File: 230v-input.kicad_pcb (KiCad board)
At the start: 2 copper layers, 61.5 x 19.8 mm, 7 parts, among them J1 PWR_IN, U1 MOC3063M, U2 LTV-814

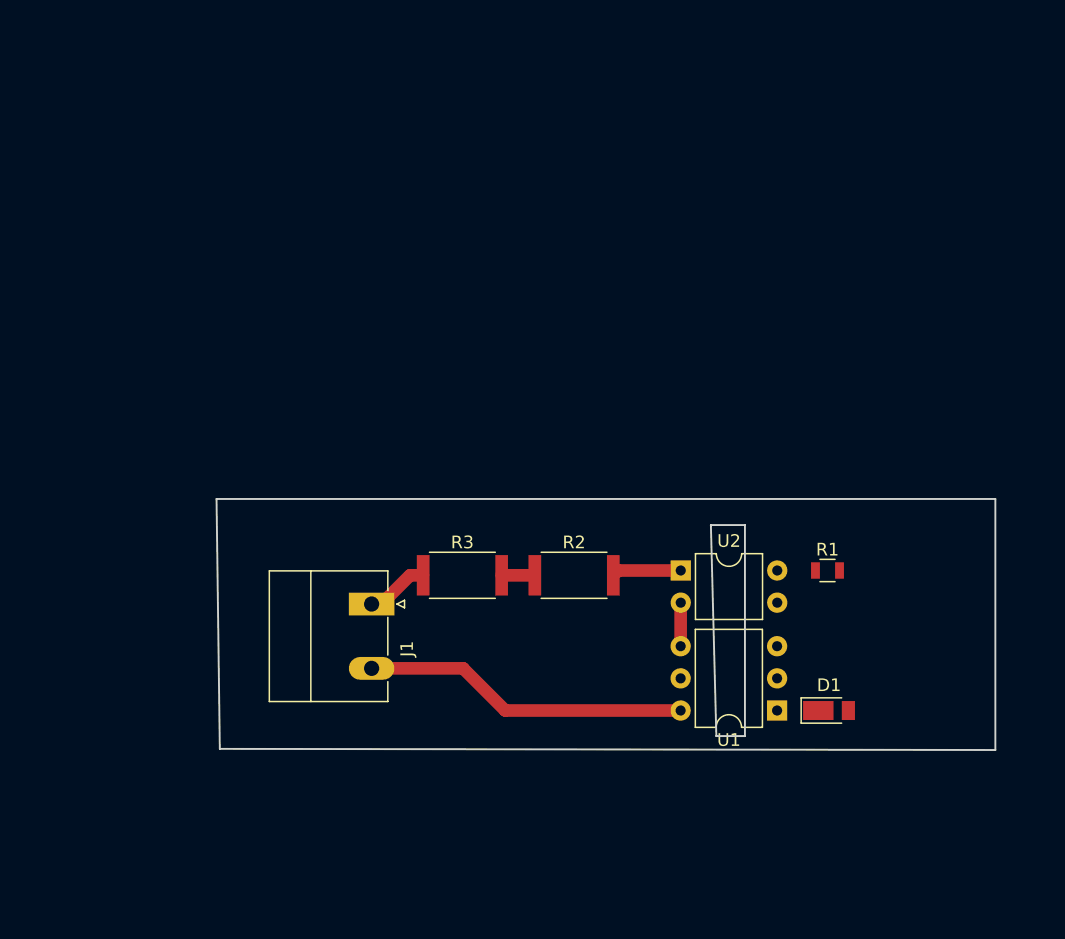
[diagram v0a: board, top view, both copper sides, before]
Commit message: Finish first rev
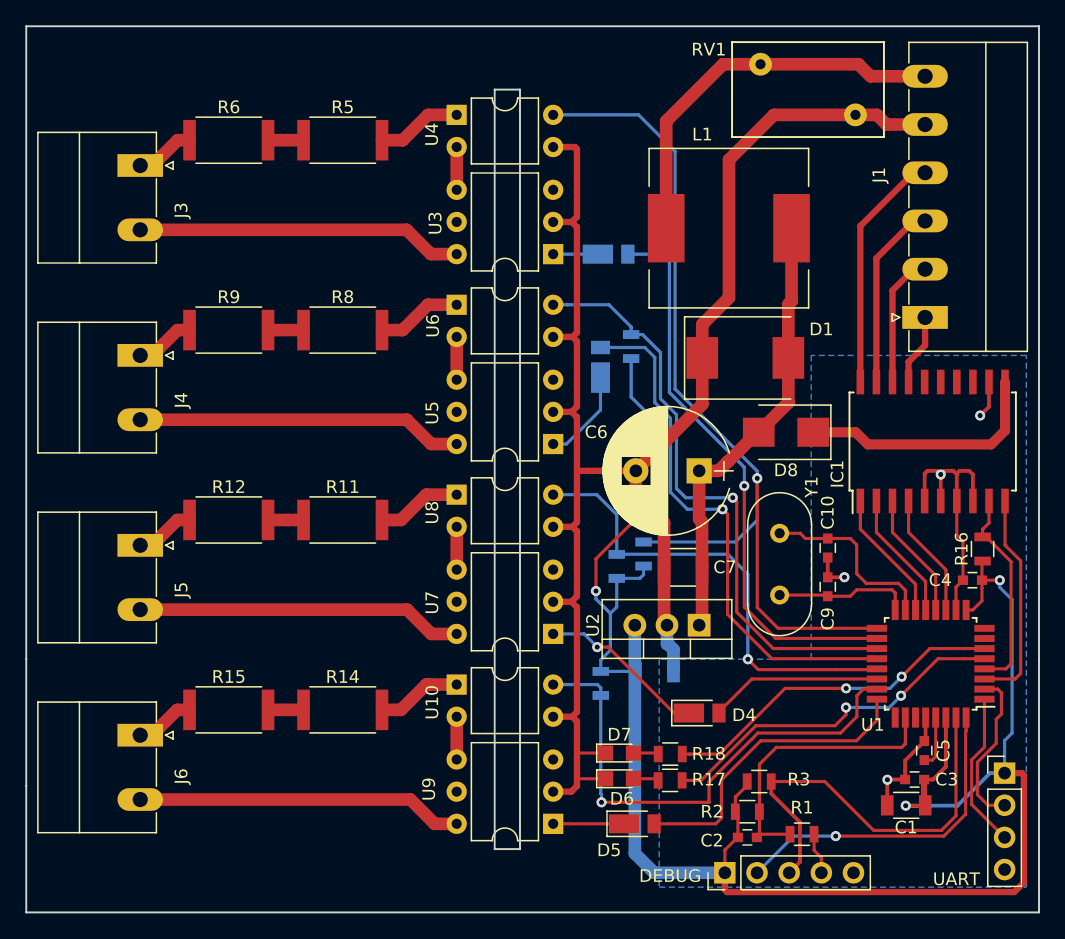
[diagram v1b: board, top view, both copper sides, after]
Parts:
- added C1: 10µF/10V, Capacitors_SMD:C_1206, F.Cu at (89.5, 81.5)
- added C10: 22pF, Capacitors_SMD:C_0603, F.Cu at (83.3, 61.2)
- added C2: 100pF, Capacitors_SMD:C_0603, F.Cu at (77.0, 84.1)
- added C3: 100nF, Capacitors_SMD:C_0603, F.Cu at (90.2, 79.5)
- added C4: 100nF, Capacitors_SMD:C_0603, F.Cu at (94.7, 63.8)
- added C5: 100nF, Capacitors_SMD:C_0603, F.Cu at (90.9, 77.2)
- added C6: 220µF/50V, Capacitors_THT:CP_Radial_D10.0mm_P5.00mm, F.Cu at (73.2, 55.1)
- added C7: 10µF/50V, Capacitors_SMD:C_1210, F.Cu at (71.9, 62.7)
- added C8: 10µF/10V, Capacitors_SMD:C_1206, B.Cu at (69.6, 71.0)
- added C9: 22pF, Capacitors_SMD:C_0603, F.Cu at (83.3, 64.3)
- added D2: AL5809-15, Diodes_SMD:D_PowerDI-123, B.Cu at (66.0, 38.0)
- added D3: AL5809-15, Diodes_SMD:D_PowerDI-123, B.Cu at (65.4, 46.9)
- added D4: AL5809-15, Diodes_SMD:D_PowerDI-123, F.Cu at (73.2, 74.2)
- added D5: AL5809-15, Diodes_SMD:D_PowerDI-123, F.Cu at (68.1, 83.0)
- added D6: LED_RD, LEDs:LED_0805, F.Cu at (66.9, 79.4)
- added D7: LED_GN, LEDs:LED_0805, F.Cu at (66.9, 77.4)
- added D8: STPS3L60U, Diodes_SMD:D_SMB, F.Cu at (80.0, 52.1)
- added IC1: UDN2987, Housings_SOIC:SOIC-20W_7.5x12.8mm_Pitch1.27mm, F.Cu at (91.6, 52.8)
- added J2: DEBUG, Pin_Headers:Pin_Header_Straight_1x05_Pitch2.54mm, F.Cu at (75.2, 86.9)
- added J3: PWR_IN, Connectors_Phoenix:PhoenixContact_MC-G_02x5.08mm_Angled, F.Cu at (29.0, 31.0)
- added J4: PWR_IN, Connectors_Phoenix:PhoenixContact_MC-G_02x5.08mm_Angled, F.Cu at (29.0, 46.0)
- added J5: PWR_IN, Connectors_Phoenix:PhoenixContact_MC-G_02x5.08mm_Angled, F.Cu at (29.0, 61.0)
- added J6: PWR_IN, Connectors_Phoenix:PhoenixContact_MC-G_02x5.08mm_Angled, F.Cu at (29.0, 76.0)
- added J7: UART, Pin_Headers:Pin_Header_Straight_1x04_Pitch2.54mm, F.Cu at (97.3, 79.0)
- added L1: DE1207-82, Inductors_SMD:L_12x12mm_h8mm, F.Cu at (75.5, 36.0)
- added R10: 4k7, Resistors_SMD:R_0805, B.Cu at (66.6, 62.7)
- added R11: 12k/1W, Resistors_SMD:R_2512, F.Cu at (45.0, 59.0)
- added R12: 12k/1W, Resistors_SMD:R_2512, F.Cu at (36.0, 59.0)
- added R13: 4k7, Resistors_SMD:R_0805, B.Cu at (65.4, 71.9)
- added R14: 12k/1W, Resistors_SMD:R_2512, F.Cu at (45.0, 74.0)
- added R15: 12k/1W, Resistors_SMD:R_2512, F.Cu at (36.0, 74.0)
- added R16: 10k, Resistors_SMD:R_0805, F.Cu at (95.5, 61.3)
- added R17: 470, Resistors_SMD:R_0805, F.Cu at (70.9, 79.6)
- added R18: 470, Resistors_SMD:R_0805, F.Cu at (70.9, 77.5)
- added R4: 4k7, Resistors_SMD:R_0805, B.Cu at (68.8, 61.7)
- added R5: 12k/1W, Resistors_SMD:R_2512, F.Cu at (45.0, 29.0)
- added R6: 12k/1W, Resistors_SMD:R_2512, F.Cu at (36.0, 29.0)
- added R7: 4k7, Resistors_SMD:R_0805, B.Cu at (67.8, 45.3)
- added R8: 12k/1W, Resistors_SMD:R_2512, F.Cu at (45.0, 44.0)
- added R9: 12k/1W, Resistors_SMD:R_2512, F.Cu at (36.0, 44.0)
- added RV1: S10K35, Varistors:RV_Disc_D12_W7.5_P7.5, F.Cu at (78.0, 23.0)
- added U10: LTV-814, Housings_DIP:DIP-4_W7.62mm, F.Cu at (54.0, 72.0)
- added U3: MOC3063M, Housings_DIP:DIP-6_W7.62mm, F.Cu at (61.6, 38.0)
- added U4: LTV-814, Housings_DIP:DIP-4_W7.62mm, F.Cu at (54.0, 27.0)
- added U5: MOC3063M, Housings_DIP:DIP-6_W7.62mm, F.Cu at (61.6, 53.0)
- added U6: LTV-814, Housings_DIP:DIP-4_W7.62mm, F.Cu at (54.0, 42.0)
- added U7: MOC3063M, Housings_DIP:DIP-6_W7.62mm, F.Cu at (61.6, 68.0)
- added U8: LTV-814, Housings_DIP:DIP-4_W7.62mm, F.Cu at (54.0, 57.0)
- added U9: MOC3063M, Housings_DIP:DIP-6_W7.62mm, F.Cu at (61.6, 83.0)
- added Y1: 8MHz, Crystals:Crystal_HC49-U_Vertical, F.Cu at (79.5, 60.0)
- D1: value AL5809-15 -> 1.5SMCJ30CA; footprint Diodes_SMD:D_PowerDI-123 -> Diodes_SMD:D_SMC
- J1: value PWR_IN -> LOGIC_OUT; footprint Connectors_Phoenix:PhoenixContact_MC-G_02x5.08mm_Angled -> Connectors_Phoenix:PhoenixContact_MC-G_06x3.81mm_Angled
- R1: value 4k7 -> 330; footprint Resistors_SMD:R_0805 -> Inductors_SMD:L_0805
- R2: value 12k/1W -> 2k2; footprint Resistors_SMD:R_2512 -> Inductors_SMD:L_0805
- R3: value 12k/1W -> 1k; footprint Resistors_SMD:R_2512 -> Inductors_SMD:L_0805
- U1: value MOC3063M -> SAMC20E18A-AU; footprint Housings_DIP:DIP-6_W7.62mm -> Housings_QFP:TQFP-32_7x7mm_Pitch0.8mm
- U2: value LTV-814 -> AMSR-7805-NZ; footprint Housings_DIP:DIP-4_W7.62mm -> TO_SOT_Packages_THT:TO-220-3_Vertical
- moved J1 49.2 mm to (91.0, 43.0), turned to 90 degrees
- moved D1 28.6 mm to (76.8, 46.2)
- moved R3 28.6 mm to (77.9, 79.7), turned to 180 degrees
- moved R2 23.2 mm to (77.0, 82.0), turned to 180 degrees
- moved R1 20.9 mm to (81.3, 83.8)
- moved U1 12.7 mm to (91.4, 70.4)
- moved U2 4.56 mm to (73.2, 67.3), turned to 180 degrees
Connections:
- D1 pad 1: Net-(D1-Pad1) -> GND
- D1 pad 2: /DETECT_TRIG -> +24V
- J1 pad 1: Net-(J1-Pad1) -> Net-(IC1-Pad17)
- J1 pad 2: Net-(J1-Pad2) -> Net-(IC1-Pad18)
- R1 pad 1: /PWR_DETECT -> Net-(C2-Pad1)
- R1 pad 2: +5V -> /MCU_RESET
- R2 pad 1: Net-(R2-Pad1) -> Net-(C2-Pad1)
- R2 pad 2: Net-(R2-Pad2) -> +5V
- R3 pad 1: Net-(J1-Pad1) -> /SWCLK
- R3 pad 2: Net-(R2-Pad1) -> +5V
- U1 pad 1: Net-(D1-Pad1) -> /UART_RX
- U1 pad 2: GND -> /UART_TX
- U1 pad 3: Net-(U1-Pad3) -> /OUT_RST
- U1 pad 4: Net-(U1-Pad4) -> /FAULT
- U1 pad 6: Net-(J1-Pad2) -> Net-(R18-Pad2)
- U2 pad 1: Net-(R2-Pad2) -> +24V
- U2 pad 2: Net-(U1-Pad4) -> GND
- U2 pad 3: GND -> +5V
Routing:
- net GND: track 0.00 -> 173.3 mm, vias 0 -> 4
- net +5V: track 0.00 -> 146.9 mm, vias 0 -> 4
- net /DETECT_A: track 0.00 -> 72.7 mm, vias 0 -> 1
- net /DETECT_B: track 0.00 -> 47.8 mm, vias 0 -> 1
- net /TRIG_A: track 0.00 -> 44.8 mm, vias 0 -> 1
- net /TRIG_B: track 0.00 -> 42.2 mm, vias 0 -> 1
- net /DETECT_D: track 0.00 -> 40.3 mm, vias 0 -> 1
- net /DETECT_C: track 0.00 -> 37.1 mm, vias 0 -> 1
- net +24V: track 0.00 -> 35.5 mm
- net /SWCLK: track 0.00 -> 32.9 mm
- net VDD: track 0.00 -> 31.2 mm
- net Net-(R17-Pad2): track 0.00 -> 28.2 mm, vias 0 -> 2
- net Net-(R18-Pad2): track 0.00 -> 27.3 mm, vias 0 -> 2
- net /SWDIO: track 0.00 -> 26.0 mm, vias 0 -> 1
- net Net-(J6-Pad2): track 0.00 -> 25.8 mm
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- added copper zone on B.Cu, net GND
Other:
- board size 61.5 x 19.8 mm -> 80 x 70 mm

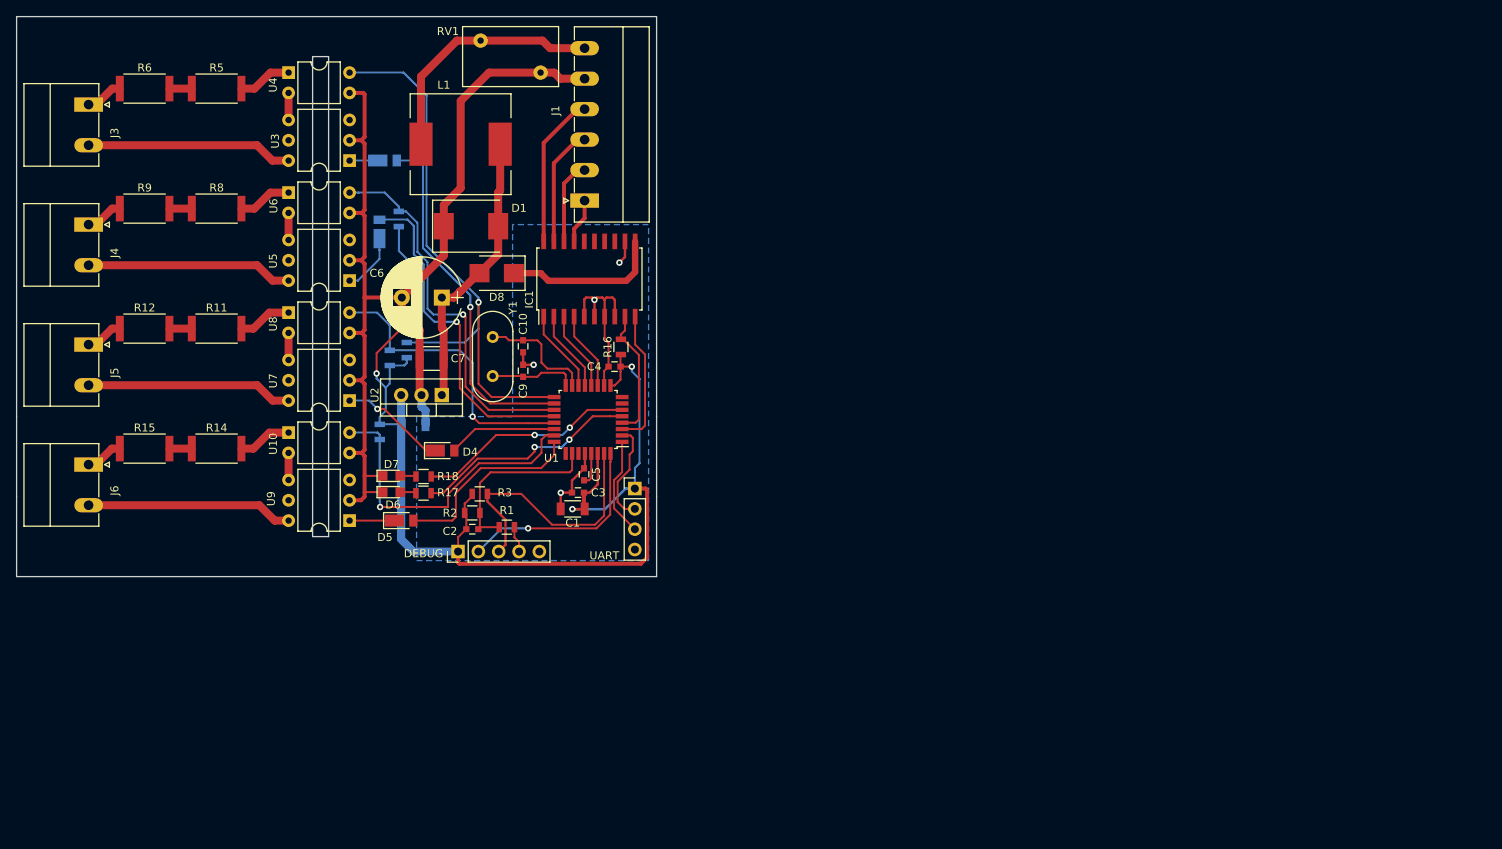
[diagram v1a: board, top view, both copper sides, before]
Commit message: Adapt to case
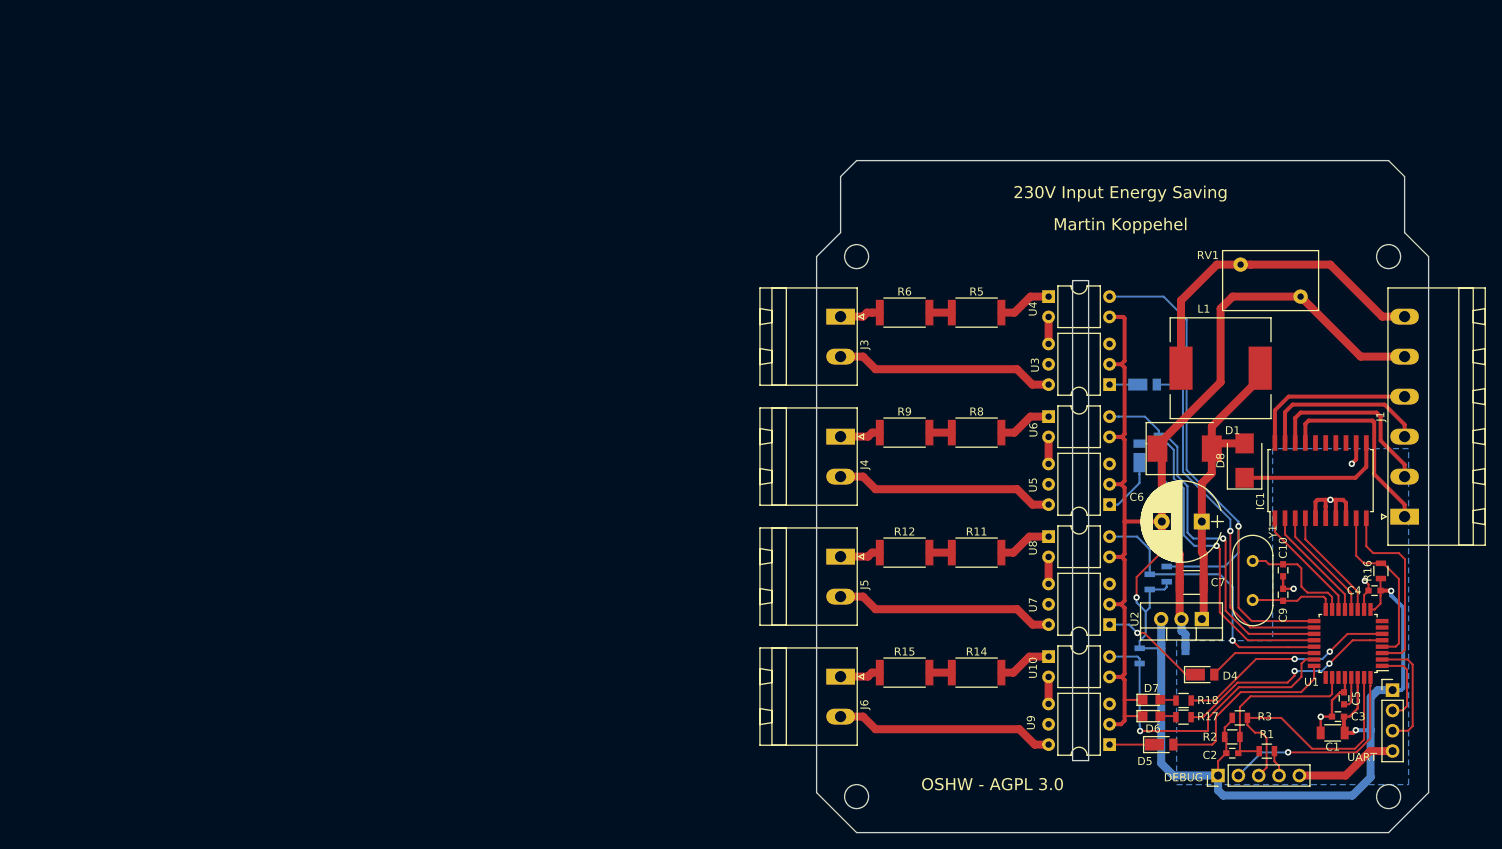
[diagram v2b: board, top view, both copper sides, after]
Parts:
- added REF**: MountingHole_3mm, Mounting_Holes:MountingHole_3mm, F.Cu at (191.5, 50.0)
- added REF**: MountingHole_3mm, Mounting_Holes:MountingHole_3mm, F.Cu at (125.0, 50.0)
- added REF**: MountingHole_3mm, Mounting_Holes:MountingHole_3mm, F.Cu at (125.0, 117.5)
- added REF**: MountingHole_3mm, Mounting_Holes:MountingHole_3mm, F.Cu at (191.5, 117.5)
- J1: footprint Connectors_Phoenix:PhoenixContact_MC-G_06x3.81mm_Angled -> Connectors_Phoenix:PhoenixContact_MSTBA-G_06x5.00mm_Angled
- J3, J4, J5, J6: footprint Connectors_Phoenix:PhoenixContact_MC-G_02x5.08mm_Angled -> Connectors_Phoenix:PhoenixContact_MSTBA-G_02x5.00mm_Angled
- moved J1 109.8 mm to (193.5, 82.5)
- moved C10 99.0 mm to (178.3, 89.2)
- moved C9 99.0 mm to (178.3, 92.3)
- moved D3 99.0 mm to (160.4, 74.9)
- moved D6 99.0 mm to (161.9, 107.4)
- moved D7 99.0 mm to (161.9, 105.4)
- moved R17 99.0 mm to (165.9, 107.6)
- moved C7 99.0 mm to (166.9, 90.7)
- moved C8 99.0 mm to (164.6, 99.0)
- moved D2 99.0 mm to (161.0, 66.0)
- moved D4 99.0 mm to (168.2, 102.2)
- moved D5 99.0 mm to (163.1, 111.0)
- moved J2 99.0 mm to (170.2, 114.9)
- moved L1 99.0 mm to (170.5, 64.0)
- moved R1 99.0 mm to (176.3, 111.8)
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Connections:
- IC1 pad 13: (no net) -> Net-(IC1-Pad13)
- IC1 pad 14: (no net) -> Net-(IC1-Pad14)
- IC1 pad 15: (no net) -> Net-(IC1-Pad15)
- IC1 pad 16: (no net) -> Net-(IC1-Pad16)
- J7 pad 2: /UART_TX -> /UART_RX
- J7 pad 3: /UART_RX -> /UART_TX
- U1 pad 25: (no net) -> Net-(U1-Pad25)
- U1 pad 27: (no net) -> Net-(U1-Pad27)
- U1 pad 7: (no net) -> Net-(U1-Pad7)
- U1 pad 8: (no net) -> Net-(U1-Pad8)
- U3 pad 3: (no net) -> Net-(U3-Pad3)
- U3 pad 5: (no net) -> Net-(U3-Pad5)
- U5 pad 3: (no net) -> Net-(U5-Pad3)
- U5 pad 5: (no net) -> Net-(U5-Pad5)
- U7 pad 3: (no net) -> Net-(U7-Pad3)
- U7 pad 5: (no net) -> Net-(U7-Pad5)
- U9 pad 3: (no net) -> Net-(U9-Pad3)
- U9 pad 5: (no net) -> Net-(U9-Pad5)
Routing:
- net GND: track 173.3 -> 193.0 mm, vias 4 -> 5
- net Net-(IC1-Pad17): track 5.64 -> 24.6 mm
- net Net-(IC1-Pad18): track 10.5 -> 23.0 mm
- net VDD: track 31.2 -> 41.0 mm
- net +5V: track 146.9 -> 138.0 mm
- net Net-(IC1-Pad19): track 14.8 -> 21.7 mm
- net /OUT_RST: track 17.2 -> 23.3 mm
- net /FAULT: track 16.4 -> 21.6 mm
- net /LV_OUT_A: track 10.4 -> 14.7 mm
- net /LV_OUT_C: track 10.0 -> 14.3 mm
- net /LV_OUT_B: track 10.2 -> 14.5 mm
- net /LV_OUT_D: track 9.83 -> 14.1 mm
- net +24V: track 35.5 -> 38.9 mm
- net /UART_RX: track 12.4 -> 9.90 mm
- net Net-(IC1-Pad20): track 19.2 -> 21.0 mm
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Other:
- board size 80 x 70 mm -> 76.5 x 84 mm
- board text added: "230V Input Energy Saving"
- board text added: "Martin Koppehel"
- board text added: "OSHW - AGPL 3.0"
